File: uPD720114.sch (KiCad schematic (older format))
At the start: 65 parts, among them U10 DLW21SN900SQ2, U11 IP4220CZ6, U13 IP4220CZ6, U15 AP2146, U16 AP2146, U17 IO_USB_A_90, U2 DLW21SN900SQ2, U22 DLW21SN900SQ2, U3 IP4220CZ6, U4 UPD720114-QFP48, U5 DLW21SN900SQ2, U8 IO_USB_A_90, U9 DLW21SN900SQ2, X1 30MHz

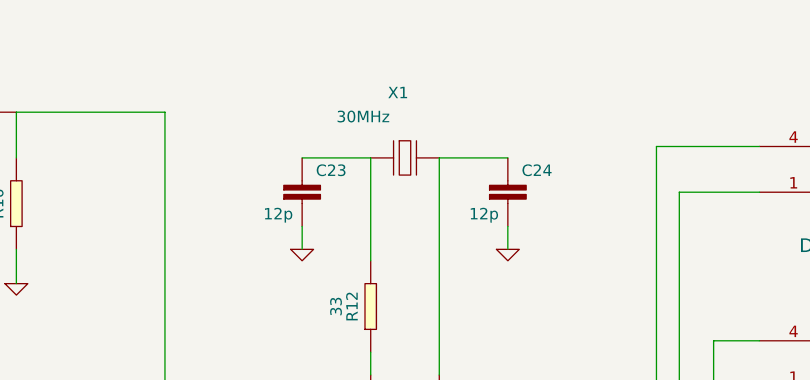
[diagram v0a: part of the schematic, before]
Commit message: 完成新要求修改，生成gerber文件
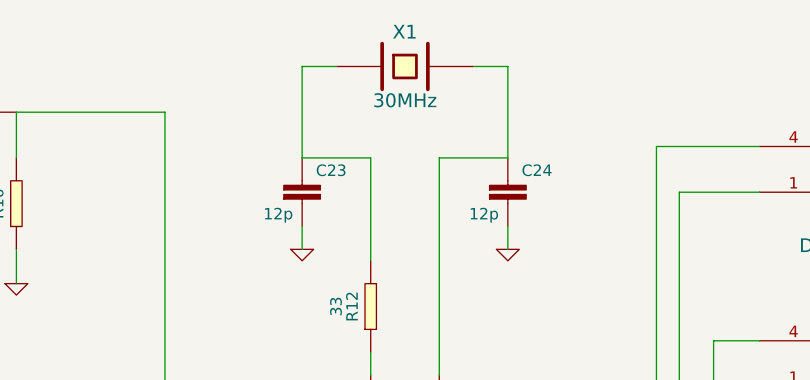
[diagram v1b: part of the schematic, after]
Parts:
- removed X1: 30MHz, C_CRY_5.0-3.2, symbol C_CRY_5.0-3.2
- added X1: 30MHz, C_CRY_DIP2, symbol C_CRY_DIP2
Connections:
- net at C24.1, U4.10 (X1): now also X1.2
- net at C23.1, R12.2: now also X1.1
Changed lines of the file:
@@
-EESchema Schematic File Version 2  date 2014/12/30 17:10:49
+EESchema Schematic File Version 2  date 2015/1/4 11:31:27
 LIBS:C
 LIBS:IC
@@
 Sheet 2 5
 Title ""
-Date "30 dec 2014"
+Date "4 jan 2015"
 Rev ""
 Comp ""
@@
 Text Label 8300 2800 2    60   ~ 0
 VBUS2
-$Comp
-L C_CRY_5.0-3.2 X1
-U 1 1 535271F7
-P 4200 1150
-F 0 "X1" H 4125 1405 50  0000 L BNN
-F 1 "30MHz" H 3900 1300 50  0000 L BNN
-F 2 "C_CRY_5.0-3.2" H 4200 800 50  0001 C CNN
-F 3 "~" H 4200 1150 60  0000 C CNN
-	1    4200 1150
-	1    0    0    -1
-$EndComp
 NoConn ~ 8200 3200
 NoConn ~ 7300 3200
@@
 Wire Wire Line
 	7350 3900 7750 3900
+$Comp
+L C_CRY_DIP2 X1
+U 1 1 54A8BA85
+P 4200 750
+F 0 "X1" H 4200 900 60  0000 C CNN
+F 1 "30MHz" H 4200 600 60  0000 C CNN
+F 2 "C_CRY_DIP2" H 4250 500 60  0001 C CNN
+F 3 "~" H 4200 750 60  0000 C CNN
+	1    4200 750
+	1    0    0    -1
+$EndComp
+Wire Wire Line
+	3900 750  3750 750
+Wire Wire Line
+	3750 750  3750 1150
+Wire Wire Line
+	4500 750  4650 750
+Wire Wire Line
+	4650 750  4650 1150
 $EndSCHEMATC
